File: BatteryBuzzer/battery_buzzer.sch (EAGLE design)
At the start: 30 parts, among them Q1 IRFML8244, Q2 IRFML8244, Q3 P-CHANNEL-MOSFETSOT23-3, Q4 P-CHANNEL-MOSFETSOT23-3, Q5 P-CHANNEL-MOSFETSOT23-3

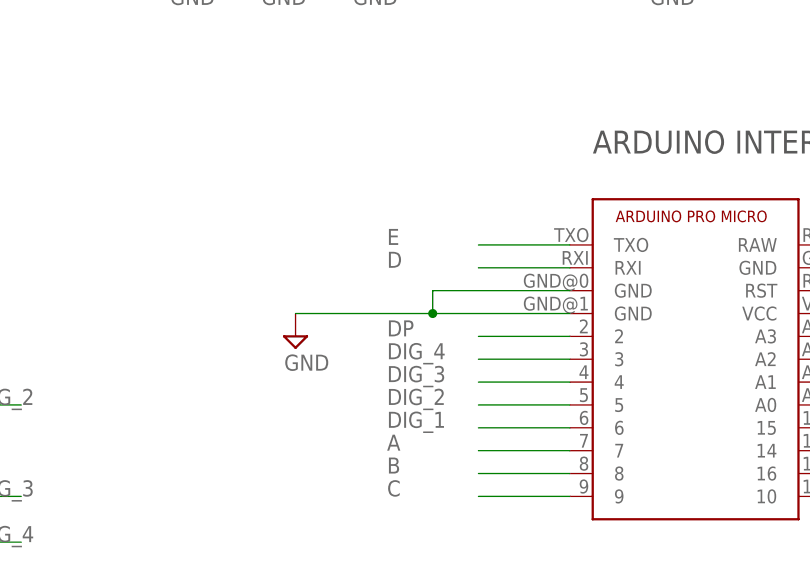
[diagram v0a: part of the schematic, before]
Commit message: and yet more pin remapping.
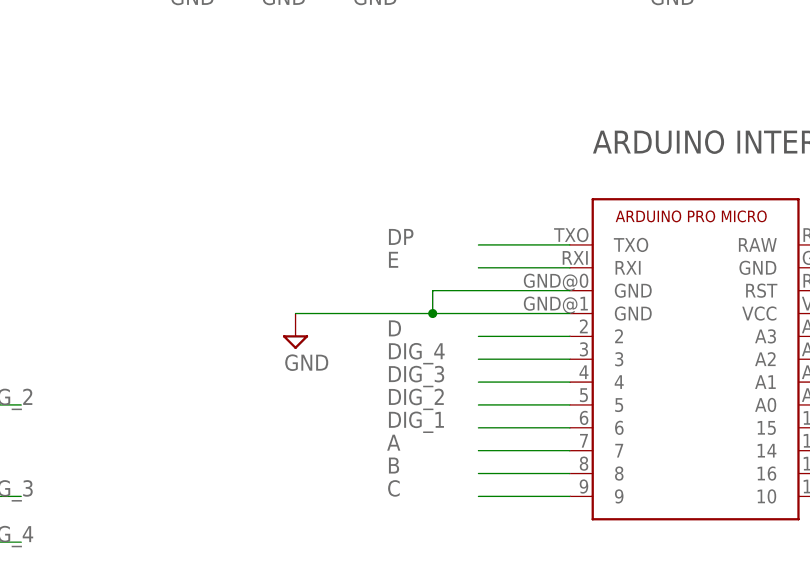
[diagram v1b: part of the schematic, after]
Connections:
- net D: now also UC1.2; no longer UC1.RXI
- net DP: now also UC1.TXO; no longer UC1.2
- net E: now also UC1.RXI; no longer UC1.TXO
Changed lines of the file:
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@@
 </segment>
 <segment>
-<pinref part="UC1" gate="G$1" pin="RXI"/>
-<wire x1="152.4" y1="73.66" x2="142.24" y2="73.66" width="0.1524" layer="91"/>
-<label x="132.08" y="73.66" size="1.778" layer="95"/>
+<pinref part="UC1" gate="G$1" pin="2"/>
+<wire x1="152.4" y1="66.04" x2="142.24" y2="66.04" width="0.1524" layer="91"/>
+<label x="132.08" y="66.04" size="1.778" layer="95"/>
 </segment>
 </net>
@@
 </segment>
 <segment>
-<pinref part="UC1" gate="G$1" pin="TXO"/>
-<wire x1="152.4" y1="76.2" x2="142.24" y2="76.2" width="0.1524" layer="91"/>
-<label x="132.08" y="76.2" size="1.778" layer="95"/>
+<pinref part="UC1" gate="G$1" pin="RXI"/>
+<wire x1="152.4" y1="73.66" x2="142.24" y2="73.66" width="0.1524" layer="91"/>
+<label x="132.08" y="73.66" size="1.778" layer="95"/>
 </segment>
 </net>
@@
 </segment>
 <segment>
-<pinref part="UC1" gate="G$1" pin="2"/>
-<wire x1="152.4" y1="66.04" x2="142.24" y2="66.04" width="0.1524" layer="91"/>
-<label x="132.08" y="66.04" size="1.778" layer="95"/>
+<pinref part="UC1" gate="G$1" pin="TXO"/>
+<wire x1="152.4" y1="76.2" x2="142.24" y2="76.2" width="0.1524" layer="91"/>
+<label x="132.08" y="76.2" size="1.778" layer="95"/>
 </segment>
 </net>
